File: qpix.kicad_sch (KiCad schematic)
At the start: 89 parts, among them J1 Conn_01x32, J13 DigReset, J2 Conn_01x09, J3 Conn_02x03, J4 Conn_02x03, J5 SPI, J6 Conn_02x03, J8 Conn_02x03, J9 Conn_Coaxial_Power, Q1 Q_NMOS_GSD, Q2 Q_NMOS_GSD, Q3 Q_NMOS_GSD, Q4 Q_NMOS_GSD, U1 qpix_digital

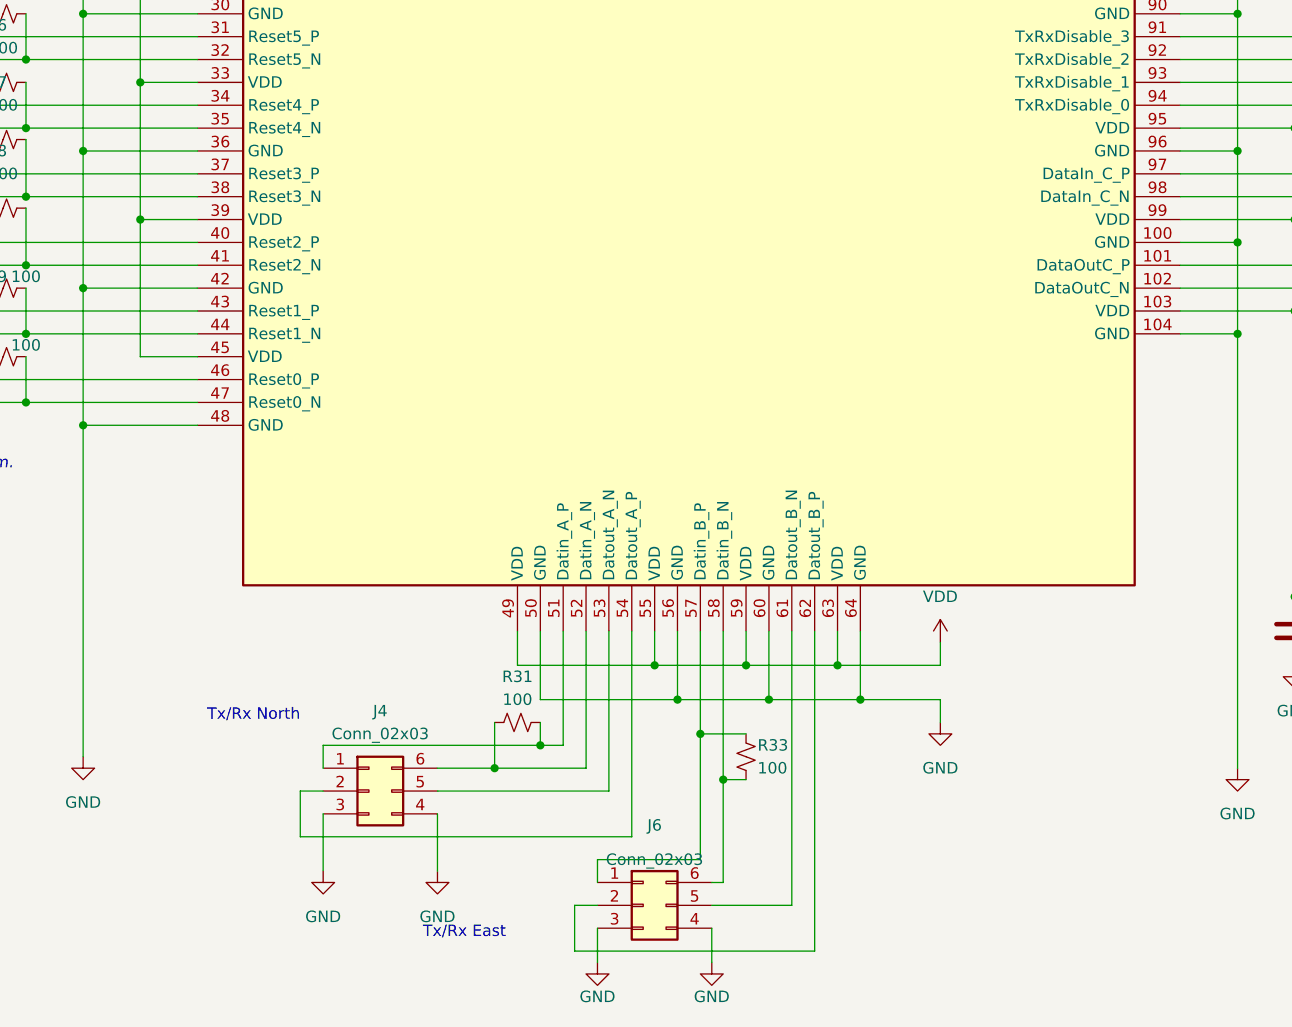
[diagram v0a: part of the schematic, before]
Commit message: some progress in routing
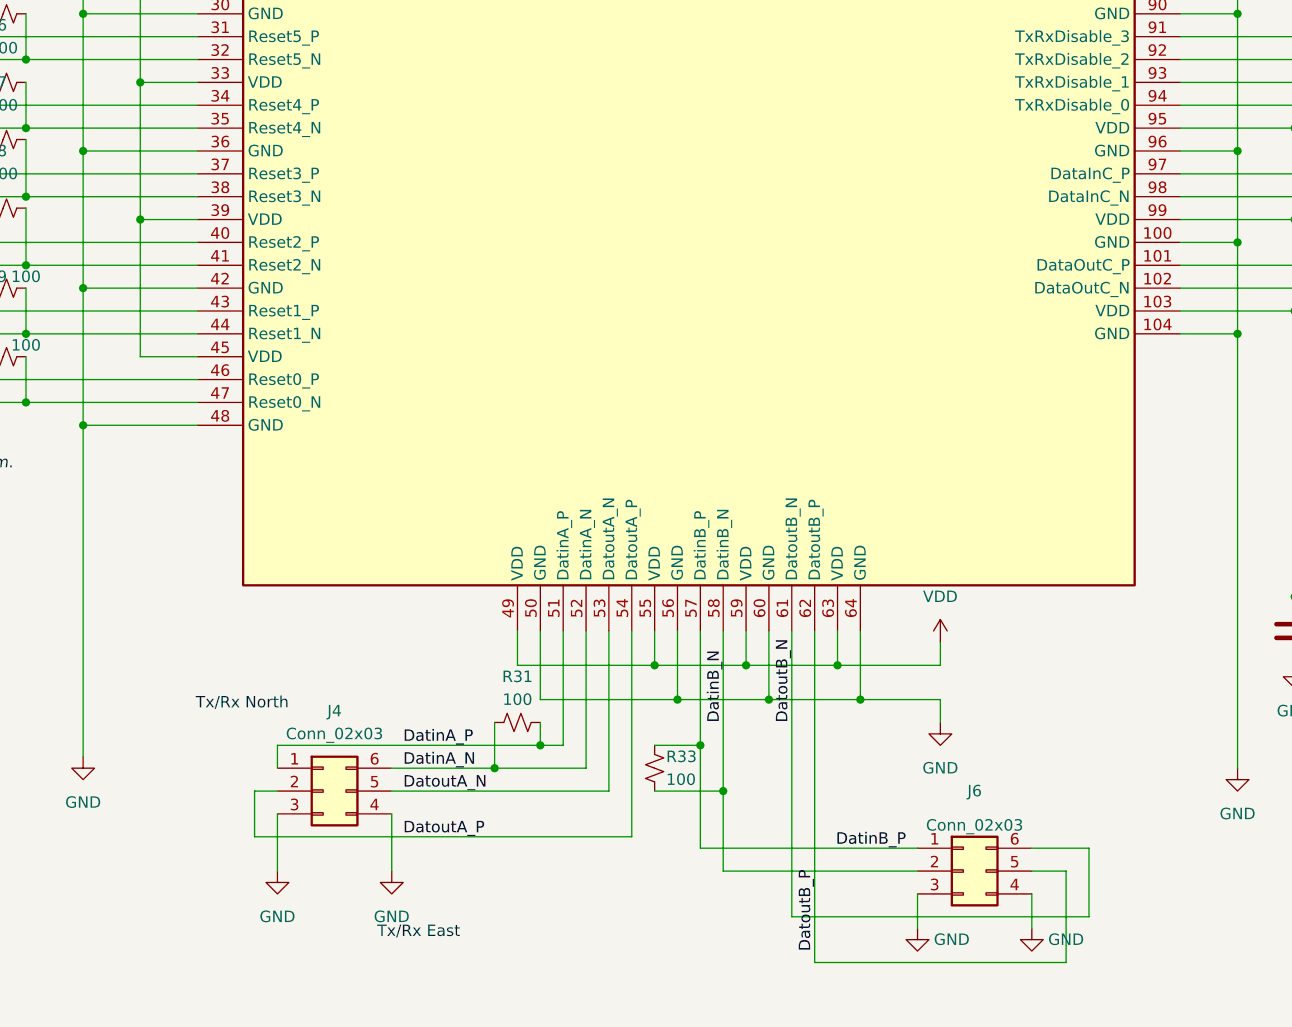
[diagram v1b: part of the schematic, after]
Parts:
- U1: footprint Package_QFP:TQFP-144_20x20mm_P0.5mm -> qpix-digi-pcb:qpix_digi_footprint
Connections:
- net DatinA_P: now reaches J4.1 (Pin_1), R31.1, U1.51 (DatinA_P)
- net DatinA_N: now reaches J4.6 (Pin_6), R31.2, U1.52 (DatinA_N)
- net DatinB_N: now reaches R33.1, U1.58 (DatinB_N)
- net DatinB_N: now also J6.2 (Pin_2); no longer J6.6 (Pin_6)
- net DatinB_P: now reaches J6.1 (Pin_1), R33.2, U1.57 (DatinB_P)
- net DatoutA_N: now reaches J4.5 (Pin_5), U1.53 (DatoutA_N)
- net DatoutA_P: now reaches J4.2 (Pin_2), U1.54 (DatoutA_P)
- net DatoutB_N: now reaches U1.61 (DatoutB_N)
- net DatoutB_N: now also J6.6 (Pin_6); no longer J6.5 (Pin_5)
- net DatoutB_P: now reaches U1.62 (DatoutB_P)
- net DatoutB_P: now also J6.5 (Pin_5); no longer J6.2 (Pin_2)
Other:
- moved on the sheet: J4, J6, R33
